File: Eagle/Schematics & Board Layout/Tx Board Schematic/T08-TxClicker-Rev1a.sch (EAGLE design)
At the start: 90 parts, among them U1 CC430F513X---RGZ48, X1-DNI SMA-SMD, Y1 26MHz

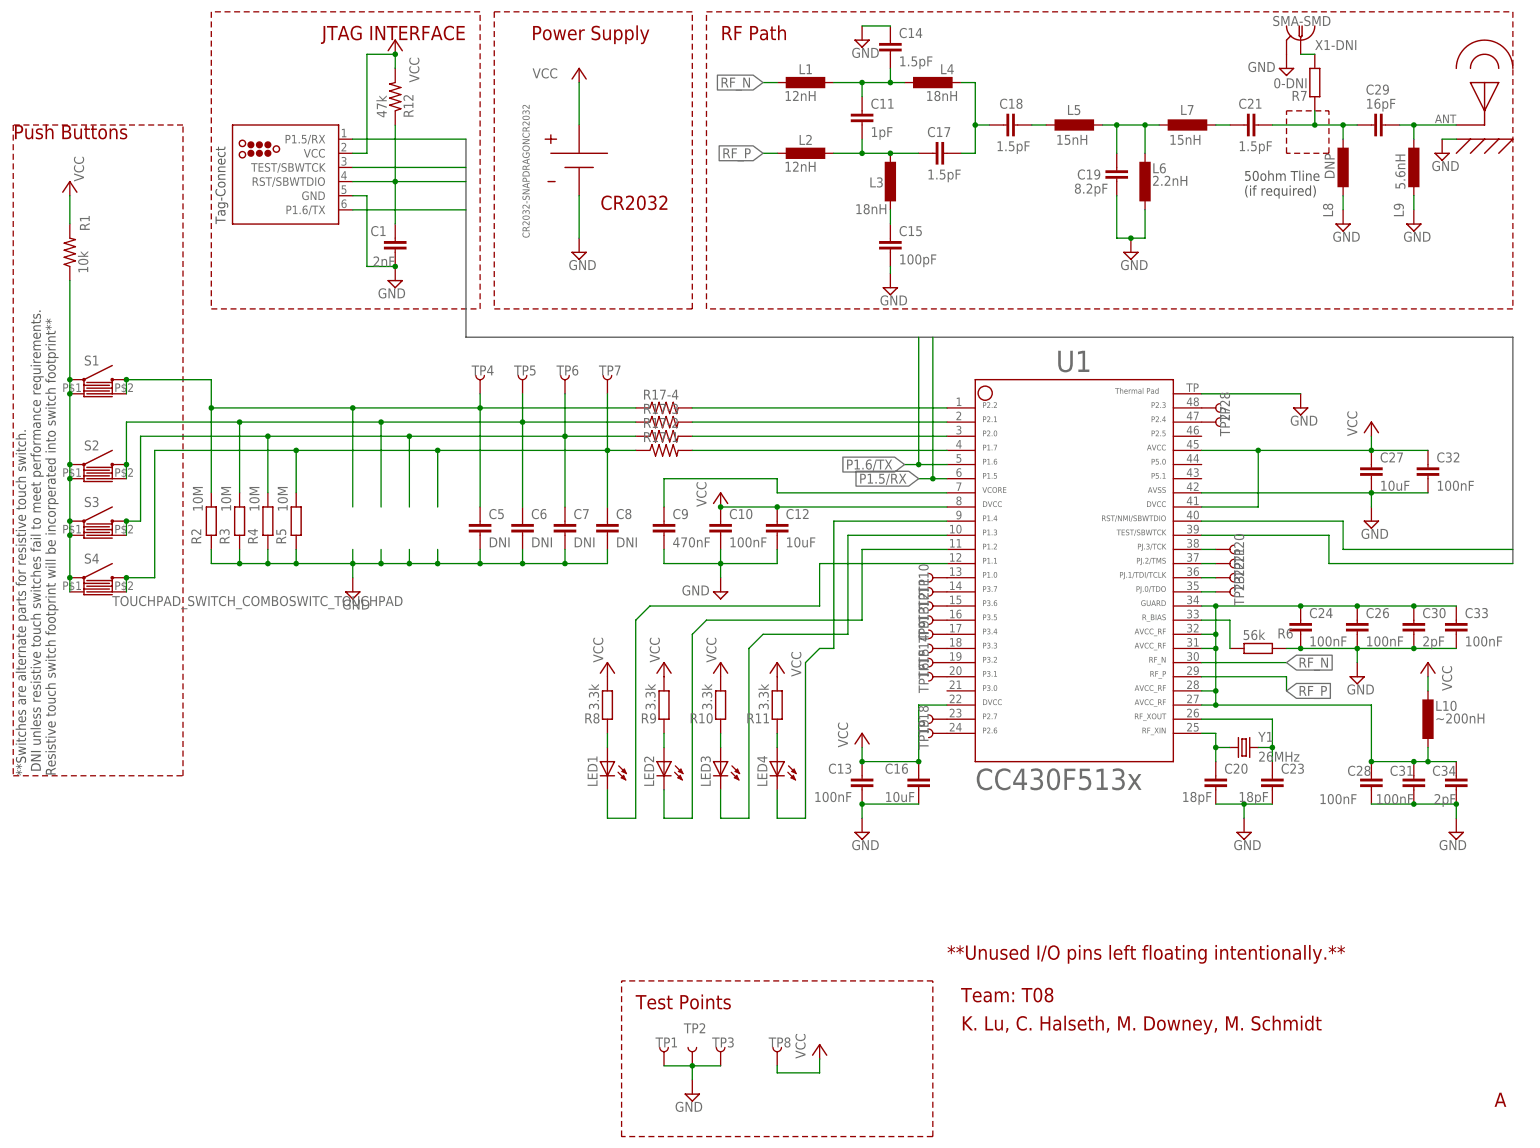
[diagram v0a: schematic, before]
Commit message: And looking decent 0.o
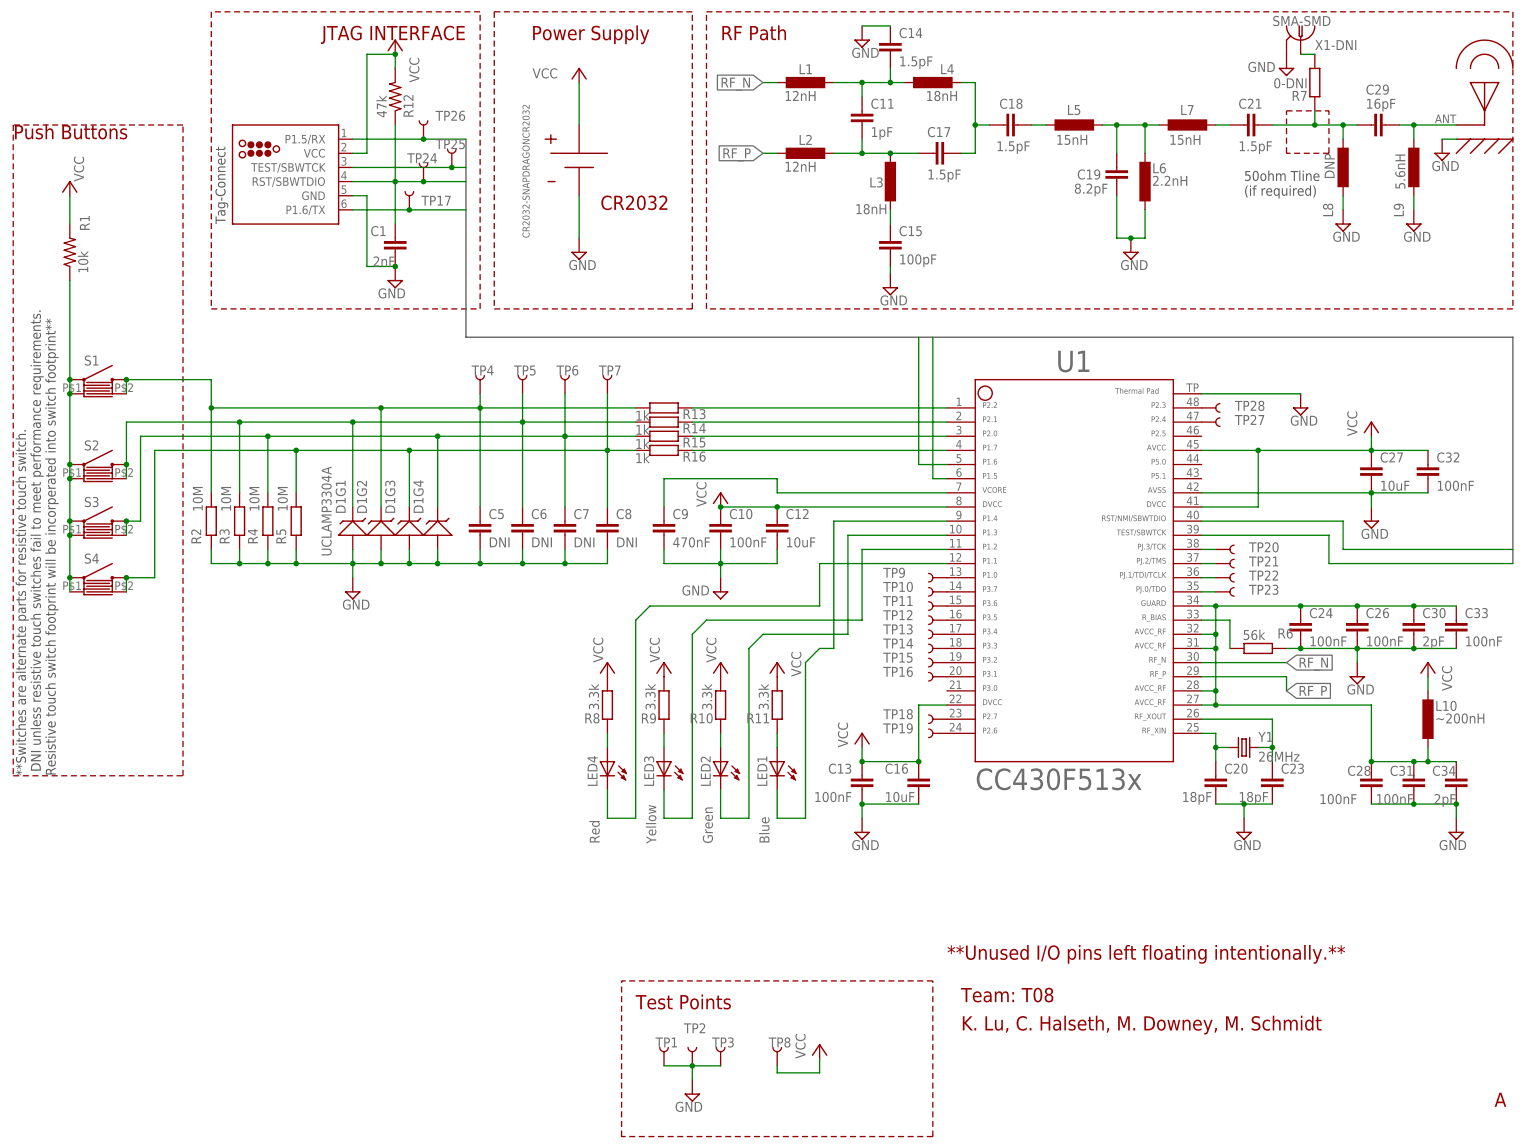
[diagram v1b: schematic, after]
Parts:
- removed R17: (no value), QuadResistor:R603X42012
- added D1: UCLAMP3304A, Semtech-TVS_Diode:UCLAMP3304A
- added R13, R14, R15, R16: 1k, rcl-amber:R0603
- added TP17, TP24, TP25, TP26: TEST-POINT3, SparkFun-Passives:TEST-POINT3
- LED1: value (none) -> Blue
- LED2: value (none) -> Green
- LED3: value (none) -> Yellow
- LED4: value (none) -> Red
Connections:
- removed net RST/SBWTDIO: C1.1, R12.1, U$1.RST/SBWTDIO
- net GND: now also D1G1.2, D1G2.2
- net N$10: now also LED2.C; no longer LED3.C
- net N$13: now also LED4.A; no longer LED1.A
- net N$14: now also LED3.A; no longer LED2.A
- net N$15: now also LED3.C; no longer LED2.C
- net N$16: now also LED2.A; no longer LED3.A
- net N$17: now also LED1.A; no longer LED4.A
- net N$18: now also LED4.C; no longer LED1.C
- net N$19: now also R14.2; no longer R17-3.2
- net N$20: now also R13.2; no longer R17-4.2
- net N$21: now also TP13.1; no longer TP9.1
- net N$22: now also TP9.1; no longer TP10.1
- net N$23: now also TP10.1; no longer TP11.1
- net N$24: now also TP11.1; no longer TP12.1
- net N$25: now also TP12.1; no longer TP13.1
- net N$7: now also R16.2; no longer R17-1.2
- net N$9: now also R15.2; no longer R17-2.2
- net P1.4: now also LED1.C; no longer LED4.C
- net P1.5/RX: now also TP26.1
- net P1.6/TX: now also TP17.1
- net P1.7: now also D1G3.P$1, R16.1; no longer R17-1.1
- net P2.0: now also D1G4.P$1, R15.1; no longer R17-2.1
- net P2.1: now also D1G1.1, R14.1; no longer R17-3.1
- net P2.2: now also D1G2.1, R13.1; no longer R17-4.1
- net RST/NMI/SBWTDIO: now also C1.1, R12.1, TP24.1, U$1.RST/SBWTDIO
- net TEST/SBWTCK: now also TP25.1
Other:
- moved on the sheet: LED1, LED2, LED3, LED4, TP10, TP11, TP12, TP13, TP9

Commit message: Move Tag Connect
Vectorized fonts, moved tag connect, added tp labels
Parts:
- TP1, TP10, TP11, TP12, TP13, TP14, TP15, TP16, TP17, TP18, TP19, TP2, TP20, TP21, TP22, TP23, TP24, TP25, TP26, TP27, TP28, TP3, TP5, TP6, TP7, TP8: value TEST-POINT3 -> (none)
- TP9: value TEST-POINT3 -> TP9
